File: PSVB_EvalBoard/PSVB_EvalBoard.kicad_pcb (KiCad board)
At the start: 2 copper layers, 456 parts, among them J10 PIN20, J11 PIN12_2x6, J12 PIN20, J13 PIN6_2x3, J2 PIN2, J29 PIN6_2x3, J3 PIN20, J30 PIN6_2x3, J31 PIN6_2x3, J4 PIN20, J5 PIN20, J6 PIN20, J7 PIN20, J8 PIN20, J9 PIN20, Q1 S9013, U1 SGM2036-ADJ, U11 93LC56BT-IOT, U12 STM32F429ZETx, U13 CH395Q, U14 CH395Q, U15 24LC64ISN, U16 MPU6050, U17 W25Q128JVSIQ, U2 SGM2036-ADJ, U3 SGM2036-ADJ, U4 INA240A1PWR, U5 INA240A1PWR, U6 TM7707, U7 REF3030, U8 REF3025, U9 REF3012, X1 2.4576Mhz, X2 12Mhz_Passive_3225, X3 16Mhz_Passive_3225, X4 30Mhz_3225, X5 30Mhz_3225

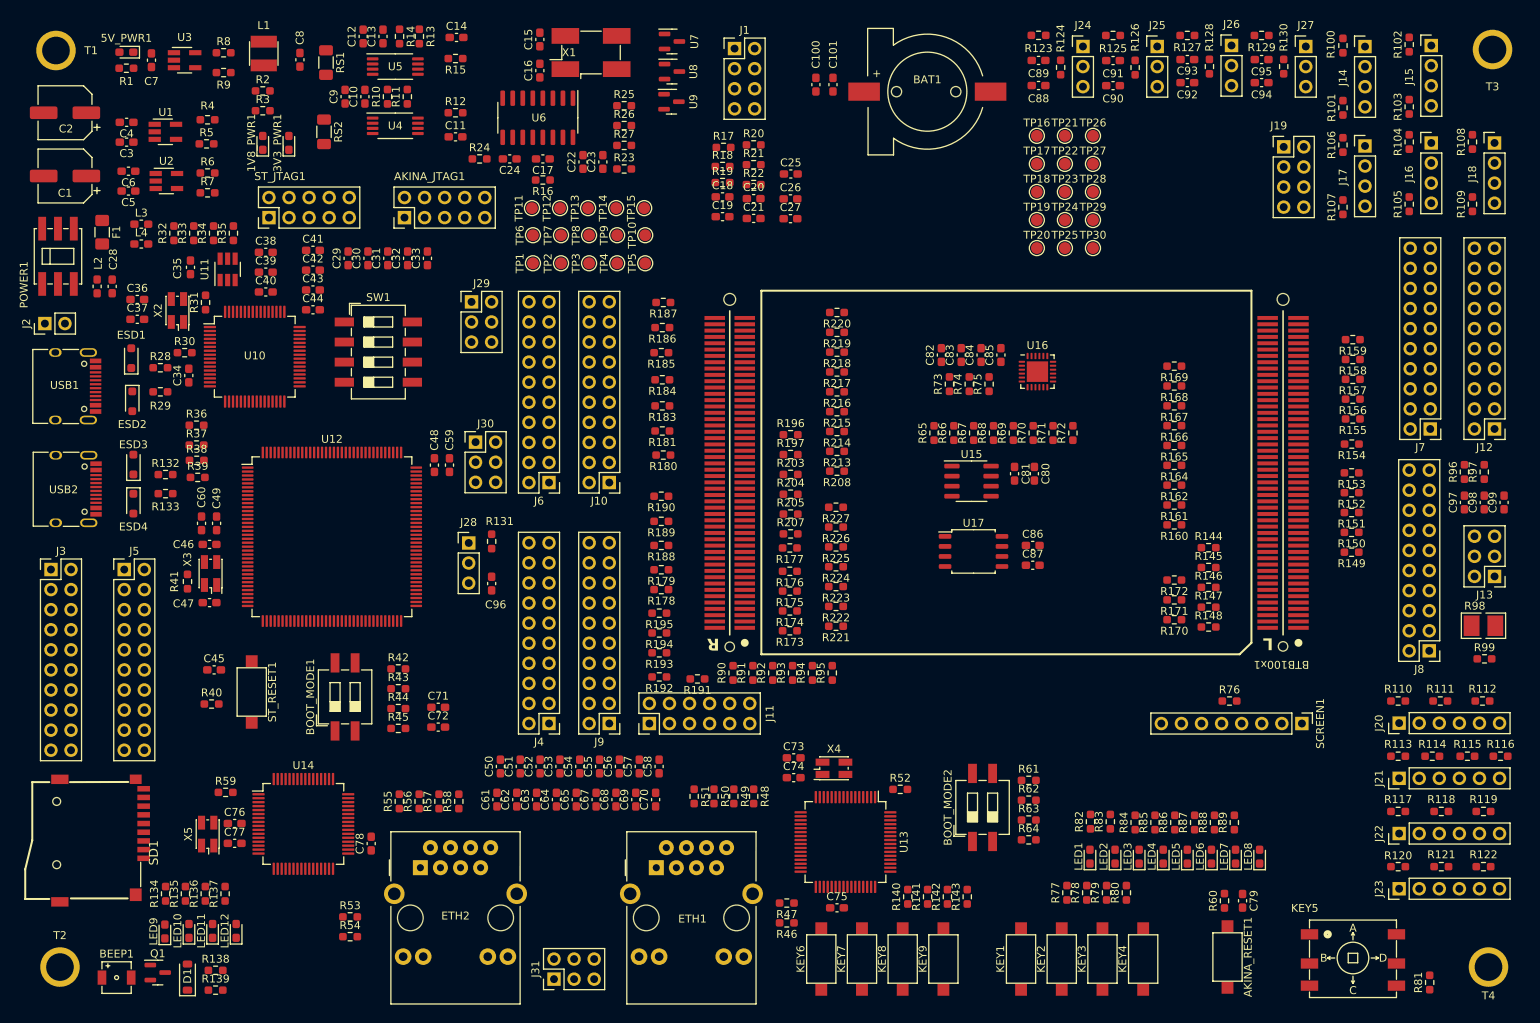
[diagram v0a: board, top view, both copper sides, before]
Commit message: Updated PCB design
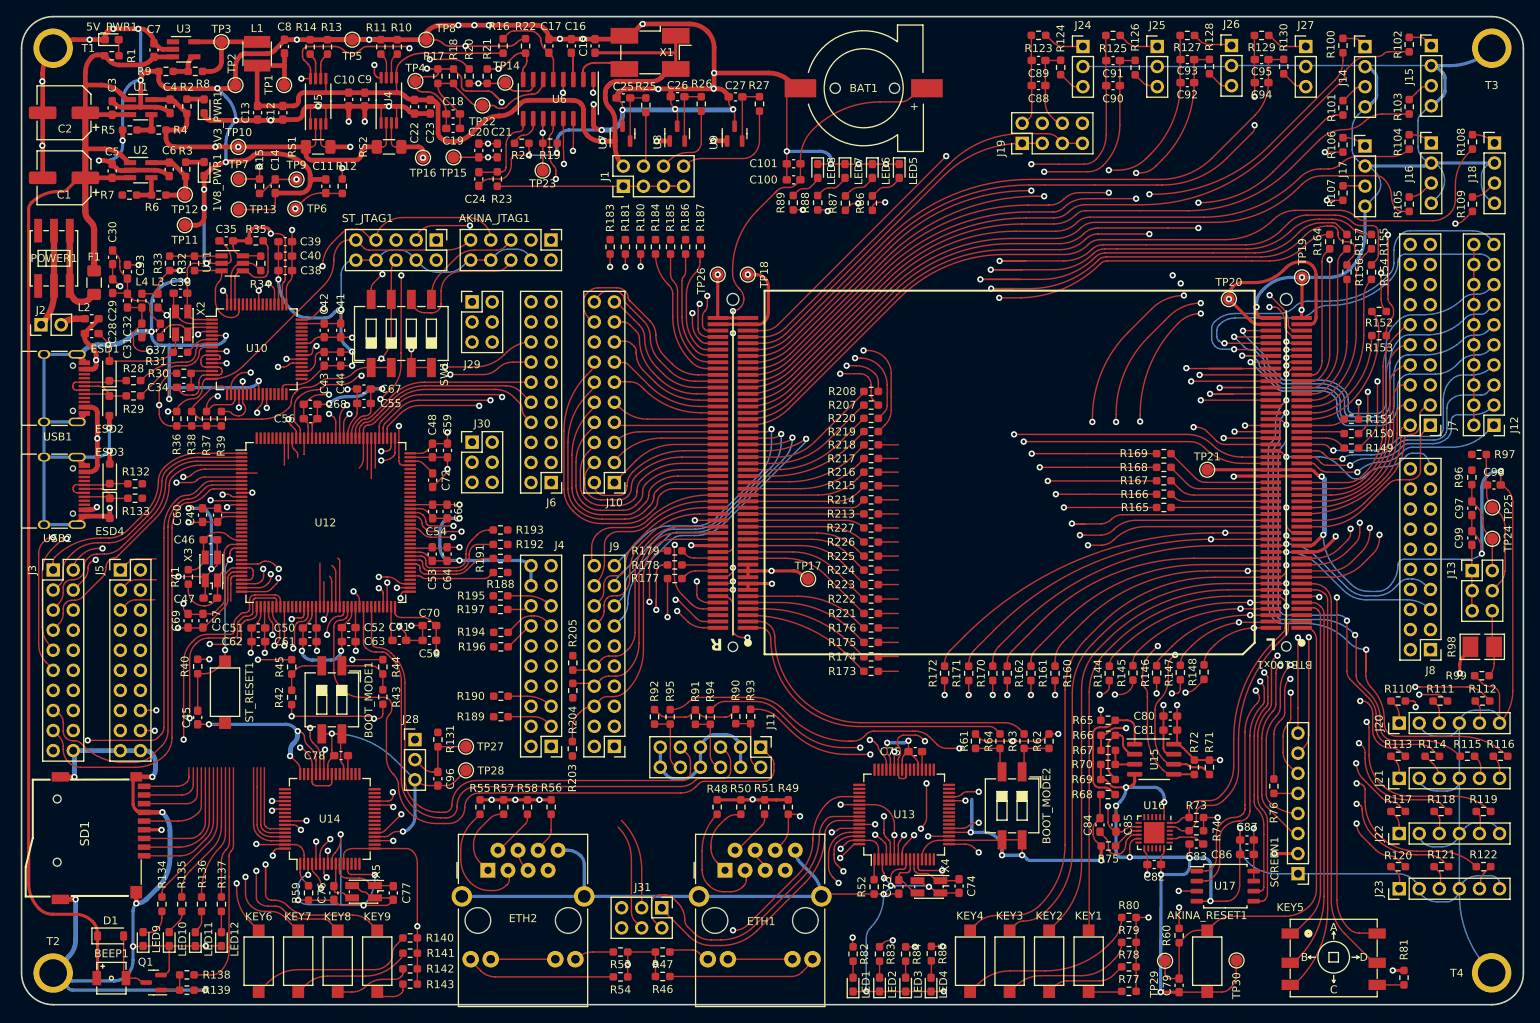
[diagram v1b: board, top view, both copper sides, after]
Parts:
- removed R158, R159: 0603 10K/1%, Resistor_SMD:R_0603_1608Metric_Pad0.98x0.95mm_HandSolder
- moved TP27 108.3 mm to (106.2, 122.4), turned to -90 degrees
- moved TP28 107.9 mm to (106.2, 125.4), turned to -90 degrees
- moved LED8 103.2 mm to (150.7, 49.5), turned to -90 degrees
- moved LED7 99.8 mm to (154.2, 49.5), turned to -90 degrees
- moved LED6 96.8 mm to (157.6, 49.5), turned to -90 degrees
- moved R89 96.2 mm to (147.6, 53.5)
- moved TP29 94.2 mm to (194.7, 149.5), turned to 90 degrees
- moved LED5 94.1 mm to (161.0, 49.5), turned to -90 degrees
- moved R88 93.1 mm to (150.7, 53.5)
- moved TP30 91.9 mm to (203.7, 149.4), turned to -90 degrees
- moved R87 90.0 mm to (154.2, 53.6)
- moved R86 87.2 mm to (157.6, 53.6)
- moved TP16 77.7 mm to (100.8, 47.9), turned to 180 degrees
- moved TP22 74.1 mm to (108.3, 41.2), turned to 180 degrees
- moved KEY9 71.6 mm to (95.0, 149.5), turned to -90 degrees
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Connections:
- net /ETH_RXN1 renamed /ETH1_RXN
- net /ETH_RXN2 renamed /ETH2_RXN
- net /ETH_RXP1 renamed /ETH1_RXP
- net /ETH_RXP2 renamed /ETH2_RXP
- net /ETH_TXN1 renamed /ETH1_TXN
- net /ETH_TXN2 renamed /ETH2_TXN
- net /ETH_TXP1 renamed /ETH1_TXP
- net /ETH_TXP2 renamed /ETH2_TXP
- BAT1 pad 2: GND -> VSS
- BTB100x1 pad 190: /EXP_PIN13 -> /BTB_PD3
- BTB100x1 pad 191: /BTB_PD3 -> /EXP_PIN13
- BTB100x1 pad 69: /BTB_PF10 -> unconnected-(BTB100x1-Pad69)
- C100 pad 2: GND -> VSS
- C101 pad 2: GND -> VSS
- C71 pad 1: VSSA -> VSS
- C72 pad 1: VSSA -> VSS
- ESD2 pad 1: Net-(ESD1-A1) -> Net-(ESD2-A1)
- J10 pad 10: /EXP_PIN9 -> /EXP_PIN8
- J10 pad 12: /EXP_PIN10 -> /BTB_PC7
- J10 pad 14: /EXP_PIN11 -> /BTB_PC6
- J10 pad 16: /EXP_PIN12 -> /EXP_PIN7
- J10 pad 2: /BTB_PC6 -> /EXP_PIN12
- J10 pad 4: /BTB_PC7 -> /EXP_PIN11
- J10 pad 6: /EXP_PIN7 -> /EXP_PIN10
- J10 pad 8: /EXP_PIN8 -> /EXP_PIN9
- J7 pad 1: /AKINA_I2C2_SCL -> /AKINA_I2C1_SCL
- J7 pad 13: unconnected-(J7-Pad13) -> /AKINA_I2C2_SCL
- J7 pad 15: unconnected-(J7-Pad15) -> /AKINA_I2C2_SDA
- J7 pad 17: /AKINA_I2C1_SCL -> unconnected-(J7-Pad17)
- J7 pad 19: /AKINA_I2C1_SDA -> unconnected-(J7-Pad19)
- J7 pad 3: /AKINA_I2C2_SDA -> /AKINA_I2C1_SDA
- R29 pad 1: Net-(USB1-A6) -> Net-(ESD2-A1)
- R63 pad 2: /AKINA_BOOT0 -> /AKINA_BOOT1
- R64 pad 2: /AKINA_BOOT1 -> /AKINA_BOOT0
- U12 pad 31: VSSA -> VSS
- U12 pad 33: +3.3VA -> +3V3
- U13 pad 22: /ETH_GPIO0 -> /ETH1_GPIO0
- U13 pad 23: /ETH_GPIO1 -> /ETH1_GPIO1
- U13 pad 24: /ETH_GPIO2 -> /ETH1_GPIO2
- U13 pad 25: /ETH_GPIO3 -> /ETH1_GPIO3
- U13 pad 26: /ETH_RST2 -> /ETH1_RST2
- U13 pad 27: /ETH_SEL -> /ETH1_SEL
- U13 pad 32: /ETH_GPIO4 -> /ETH1_GPIO4
- U13 pad 33: /ETH_GPIO5 -> /ETH1_GPIO5
- U13 pad 34: /ETH_GPIO6 -> /ETH1_GPIO6
- U13 pad 35: /ETH_GPIO7 -> /ETH1_GPIO7
- U14 pad 22: /ETH_GPIO0 -> /ETH2_GPIO0
- U14 pad 23: /ETH_GPIO1 -> /ETH2_GPIO1
- U14 pad 24: /ETH_GPIO2 -> /ETH2_GPIO2
- U14 pad 25: /ETH_GPIO3 -> /ETH2_GPIO3
- U14 pad 26: /ETH_RST2 -> /ETH2_RST2
- U14 pad 27: /ETH_SEL -> /ETH2_SEL
- U14 pad 32: /ETH_GPIO4 -> /ETH2_GPIO4
- U14 pad 33: /ETH_GPIO5 -> /ETH2_GPIO5
- U14 pad 34: /ETH_GPIO6 -> /ETH2_GPIO6
- U14 pad 35: /ETH_GPIO7 -> /ETH2_GPIO7
- USB1 pad 6: Net-(USB1-A6) -> Net-(ESD2-A1)
- USB1 pad 8: Net-(USB1-A6) -> Net-(ESD2-A1)
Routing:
- net VSS: track 0.00 -> 1745.2 mm, vias 0 -> 118
- net +3V3: track 0.00 -> 848.3 mm, vias 0 -> 56
- net +1V8: track 0.00 -> 216.5 mm, vias 0 -> 14
- net /DUT_+3.3V_1: track 0.00 -> 197.6 mm, vias 0 -> 5
- net +5V: track 0.00 -> 178.6 mm, vias 0 -> 1
- net /DUT_VDDA_3.3V_1: track 0.00 -> 168.6 mm, vias 0 -> 2
- net /AKINA_HALL_CH3: track 0.00 -> 151.9 mm, vias 0 -> 4
- net /AKINA_HALL_CH2: track 0.00 -> 143.4 mm, vias 0 -> 4
- net +3.3VA: track 0.00 -> 139.8 mm, vias 0 -> 3
- net /AKINA_USART1_TX: track 0.00 -> 133.5 mm, vias 0 -> 1
- net /AKINA_HALL_CH1: track 0.00 -> 132.3 mm, vias 0 -> 4
- net /AKINA_USART1_RX: track 0.00 -> 129.7 mm, vias 0 -> 1
- net /AKINA_CMP2_IN: track 0.00 -> 110.9 mm, vias 0 -> 2
- net /MC_BKIN_0: track 0.00 -> 107.4 mm
- net /MC_BKIN_1: track 0.00 -> 103.7 mm, vias 0 -> 2
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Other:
- board outline added: 190 x 125 mm
- copper layers 2 -> 4
